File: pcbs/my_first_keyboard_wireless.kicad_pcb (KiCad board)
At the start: 2 copper layers, 135.9 x 108 mm, 78 parts

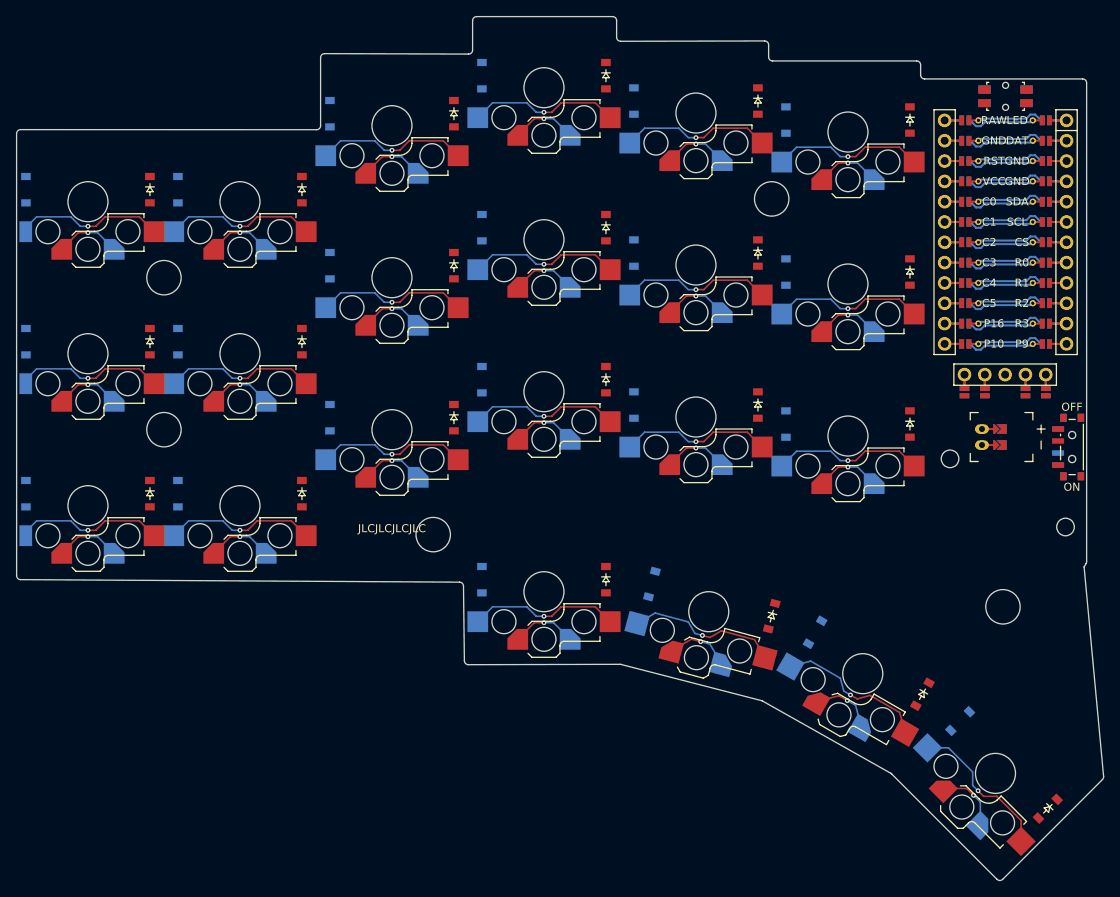
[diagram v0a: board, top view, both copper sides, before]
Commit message: v1
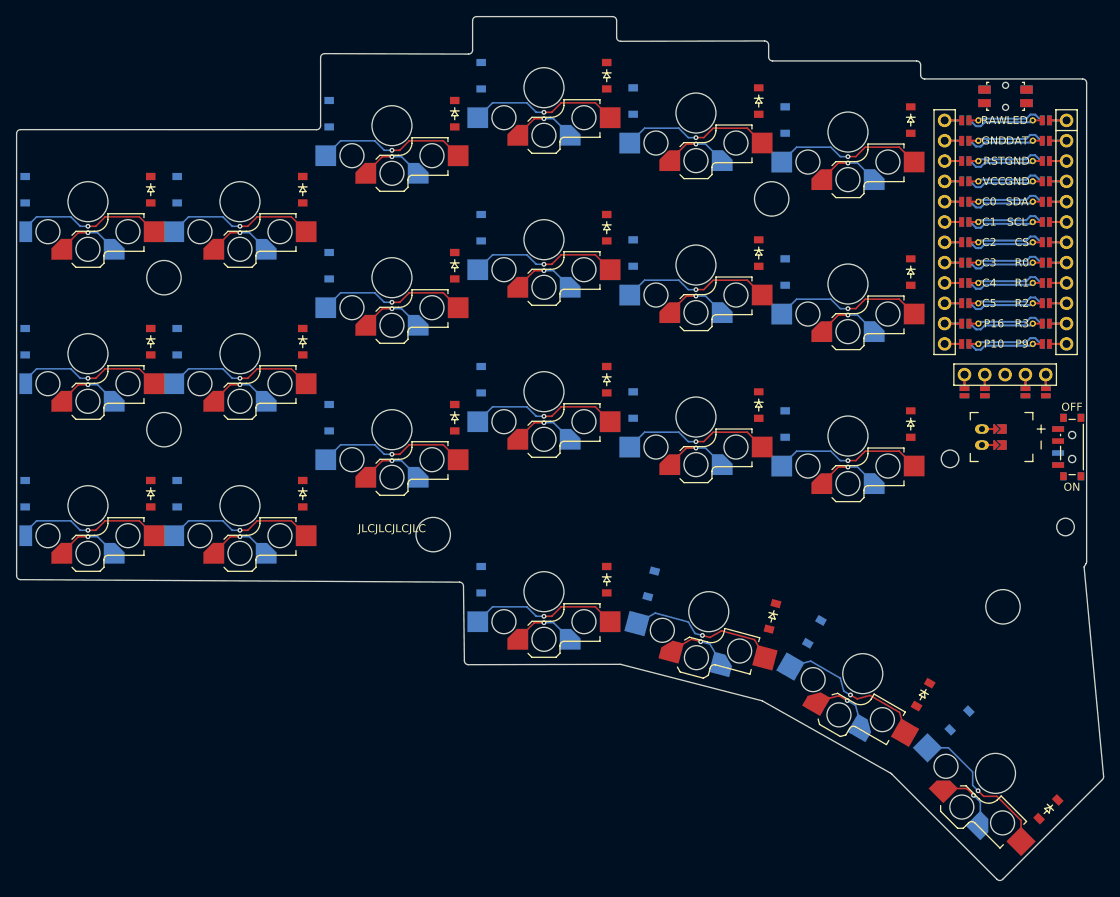
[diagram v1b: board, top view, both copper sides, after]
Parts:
- moved D44 0.10 mm to (220.1, 138.0)
- moved D21 0.10 mm to (190.8, 115.8)
- moved D43 0.10 mm to (204.4, 123.6)
- moved D1 0.10 mm to (92.2, 98.5)
- moved D10 0.10 mm to (149.2, 84.2)
- moved D11 0.10 mm to (149.2, 65.2)
- moved D12 0.10 mm to (149.2, 46.2)
- moved D13 0.10 mm to (168.2, 87.4)
- moved D14 0.10 mm to (168.2, 68.4)
- moved D15 0.10 mm to (168.2, 49.4)
- moved D16 0.10 mm to (187.2, 89.8)
- moved D17 0.10 mm to (187.2, 70.8)
- moved D18 0.10 mm to (187.2, 51.8)
- moved D19 0.10 mm to (149.2, 109.2)
- moved D2 0.10 mm to (92.2, 79.5)
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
